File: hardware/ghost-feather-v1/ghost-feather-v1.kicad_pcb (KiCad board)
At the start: 4 copper layers, 106.6 x 106.7 mm, 72 parts, among them J1 Conn_ARM_SWD_TagConnect_TC2030, J2 USB_C_Receptacle_USB2.0, J3 Conn_01x03, J4 Conn_01x03, J5 Conn_01x03, J6 Conn_01x03, J7 Conn_01x08, Q1 BSS138, Q2 BSS138, Q3 BSS138, Q4 BSS138, SW2 BOOT0, U1 STM32F722RETx, U2 BMI270, U3 USBLC6-2SC6_MOD, U4 MPM3610, U5 MPM3610, X1 16MHz, X2 32kHz768

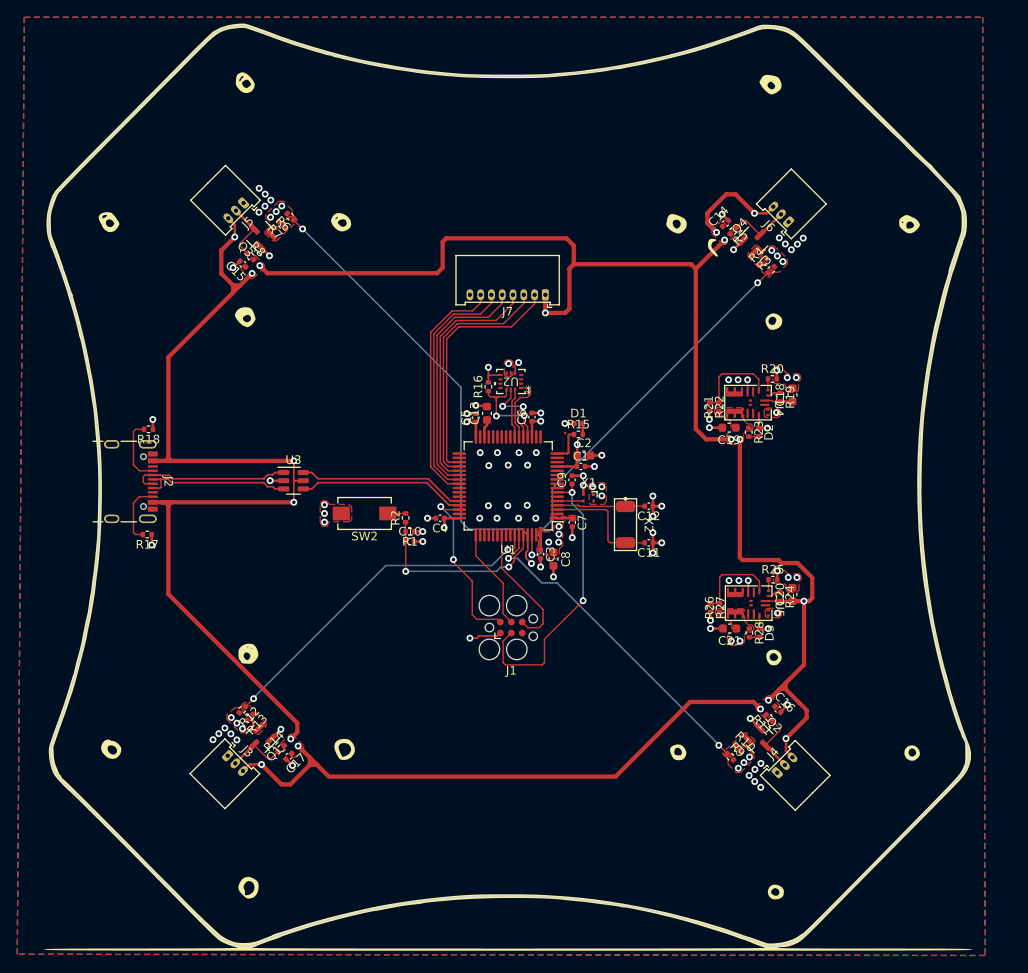
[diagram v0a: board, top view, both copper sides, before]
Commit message: feat: PCB routing #8. PCB cleanup #1
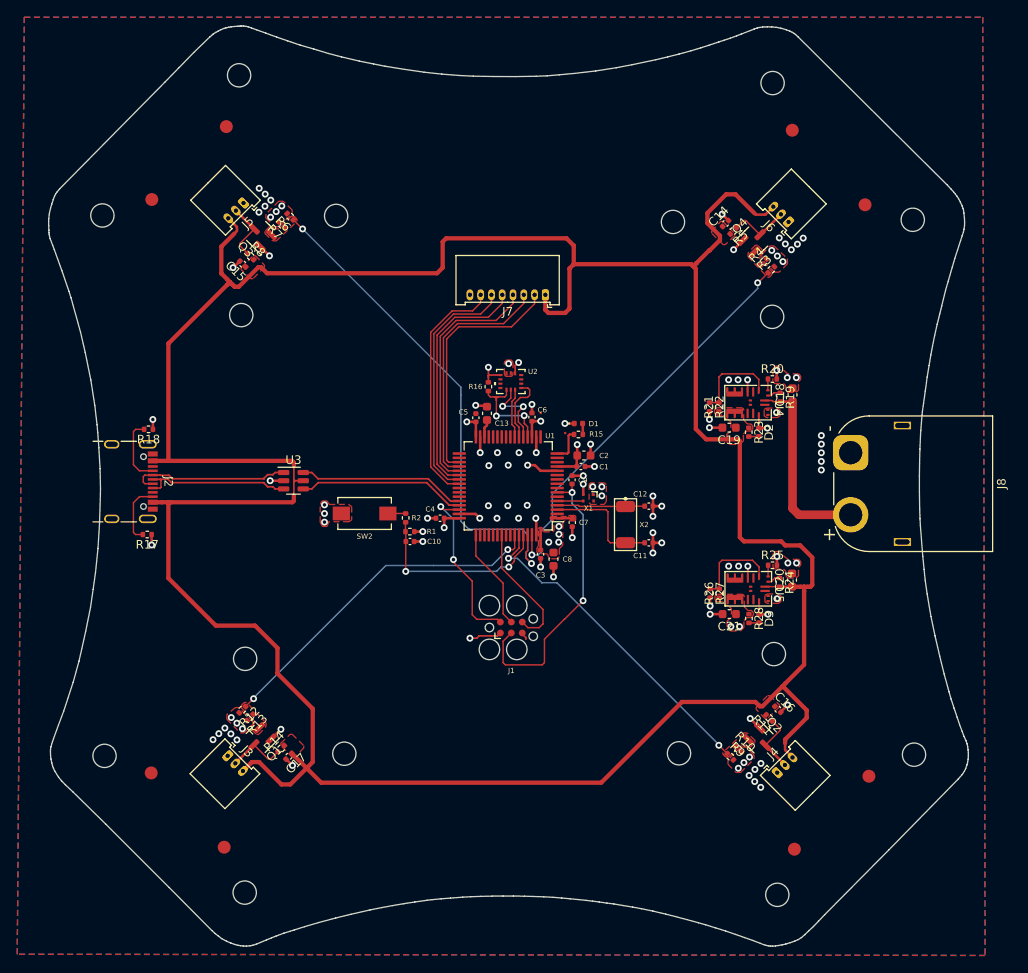
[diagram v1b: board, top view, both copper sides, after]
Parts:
- removed G***: LOGO, ghost-feather-v1:f450_04192025
- added FID1: Fiducial, Fiducial:Fiducial_1.5mm_Mask4.5mm, F.Cu at (101.2, 58.7)
- added FID2: Fiducial, Fiducial:Fiducial_1.5mm_Mask4.5mm, F.Cu at (109.8, 50.2)
- added FID3: Fiducial, Fiducial:Fiducial_1.5mm_Mask4.5mm, F.Cu at (175.4, 50.7)
- added FID4: Fiducial, Fiducial:Fiducial_1.5mm_Mask4.5mm, F.Cu at (183.9, 59.3)
- added FID5: Fiducial, Fiducial:Fiducial_1.5mm_Mask4.5mm, F.Cu at (184.3, 125.6)
- added FID6: Fiducial, Fiducial:Fiducial_1.5mm_Mask4.5mm, F.Cu at (175.7, 134.0)
- added FID7: Fiducial, Fiducial:Fiducial_1.5mm_Mask4.5mm, F.Cu at (109.6, 133.8)
- added FID8: Fiducial, Fiducial:Fiducial_1.5mm_Mask4.5mm, F.Cu at (101.1, 125.2)
- added H1: MountingHole, MountingHole:MountingHole_2.7mm_M2.5, F.Cu at (95.5, 60.5)
- added H10: MountingHole, MountingHole:MountingHole_2.7mm_M2.5, F.Cu at (173.7, 139.3)
- added H11: MountingHole, MountingHole:MountingHole_2.7mm_M2.5, F.Cu at (162.3, 122.9)
- added H12: MountingHole, MountingHole:MountingHole_2.7mm_M2.5, F.Cu at (173.3, 111.4)
- added H13: MountingHole, MountingHole:MountingHole_2.7mm_M2.5, F.Cu at (112.0, 139.1)
- added H14: MountingHole, MountingHole:MountingHole_2.7mm_M2.5, F.Cu at (95.7, 123.2)
- added H15: MountingHole, MountingHole:MountingHole_2.7mm_M2.5, F.Cu at (112.0, 112.0)
- added H16: MountingHole, MountingHole:MountingHole_2.7mm_M2.5, F.Cu at (123.5, 123.0)
- added H2: MountingHole, MountingHole:MountingHole_2.7mm_M2.5, F.Cu at (111.3, 44.3)
- added H3: MountingHole, MountingHole:MountingHole_2.7mm_M2.5, F.Cu at (122.5, 60.6)
- added H4: MountingHole, MountingHole:MountingHole_2.7mm_M2.5, F.Cu at (111.5, 72.1)
- added H5: MountingHole, MountingHole:MountingHole_2.7mm_M2.5, F.Cu at (173.2, 45.2)
- added H6: MountingHole, MountingHole:MountingHole_2.7mm_M2.5, F.Cu at (189.4, 61.0)
- added H7: MountingHole, MountingHole:MountingHole_2.7mm_M2.5, F.Cu at (173.1, 72.3)
- added H8: MountingHole, MountingHole:MountingHole_2.7mm_M2.5, F.Cu at (161.6, 61.3)
- added H9: MountingHole, MountingHole:MountingHole_2.7mm_M2.5, F.Cu at (189.5, 123.1)
- added J8: Conn_01x02, Connector_AMASS:AMASS_XT60PW-M_1x02_P7.20mm_Horizontal, F.Cu at (182.2, 88.0)
- moved C21 1.67 mm to (168.1, 106.8)
- moved R24 1.67 mm to (173.9, 103.1)
- moved R26 1.67 mm to (167.0, 104.4)
- moved R28 1.67 mm to (170.4, 107.3)
- moved C20 1.67 mm to (175.4, 102.8)
- moved D3 1.67 mm to (171.6, 107.3)
- moved R25 1.67 mm to (173.1, 101.1)
- moved R27 1.67 mm to (165.9, 104.3)
- moved U5 1.67 mm to (170.0, 103.8)
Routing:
- net +BATT: track 3.27 -> 22.7 mm
- net GND: track 45.8 -> 57.6 mm, vias 82 -> 86
- net +5V: track 346.4 -> 352.3 mm, vias 18 -> 0
